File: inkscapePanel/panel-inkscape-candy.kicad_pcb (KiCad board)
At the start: 2 copper layers, 99.9 x 38.9 mm, 39 parts

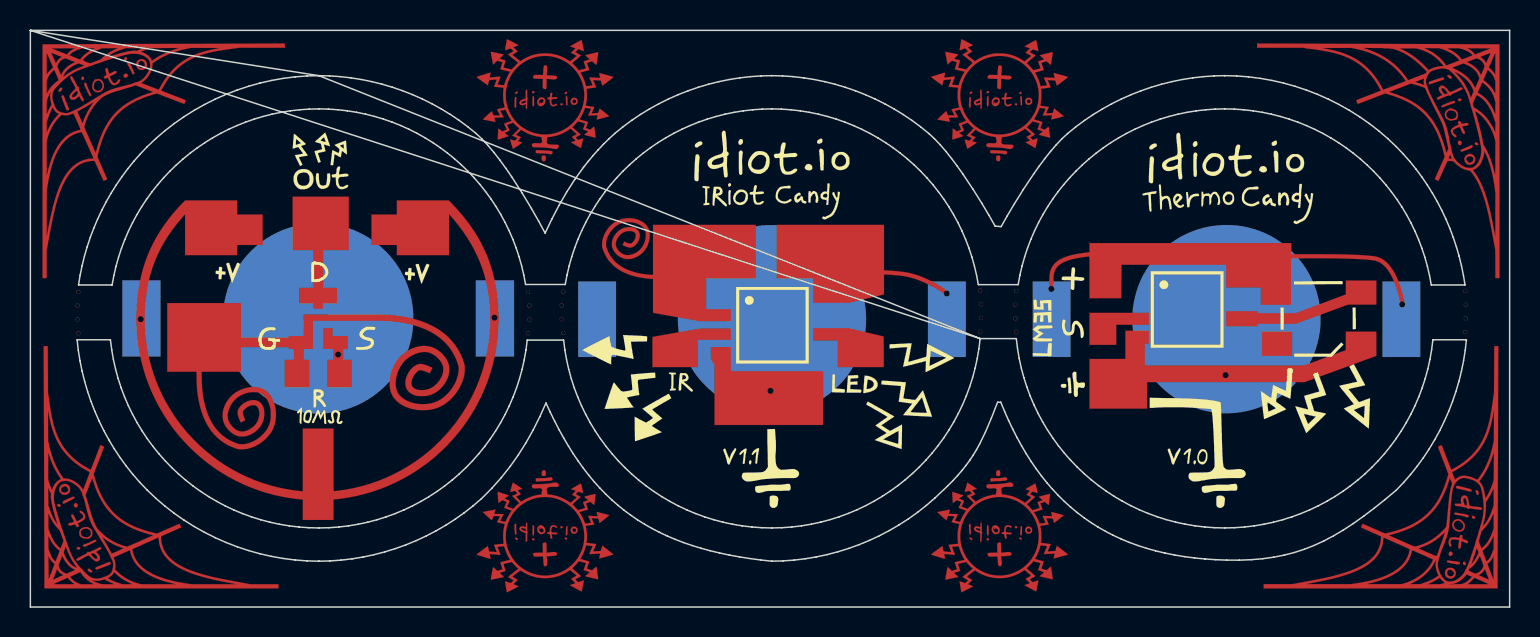
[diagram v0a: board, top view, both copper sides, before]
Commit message: new panel
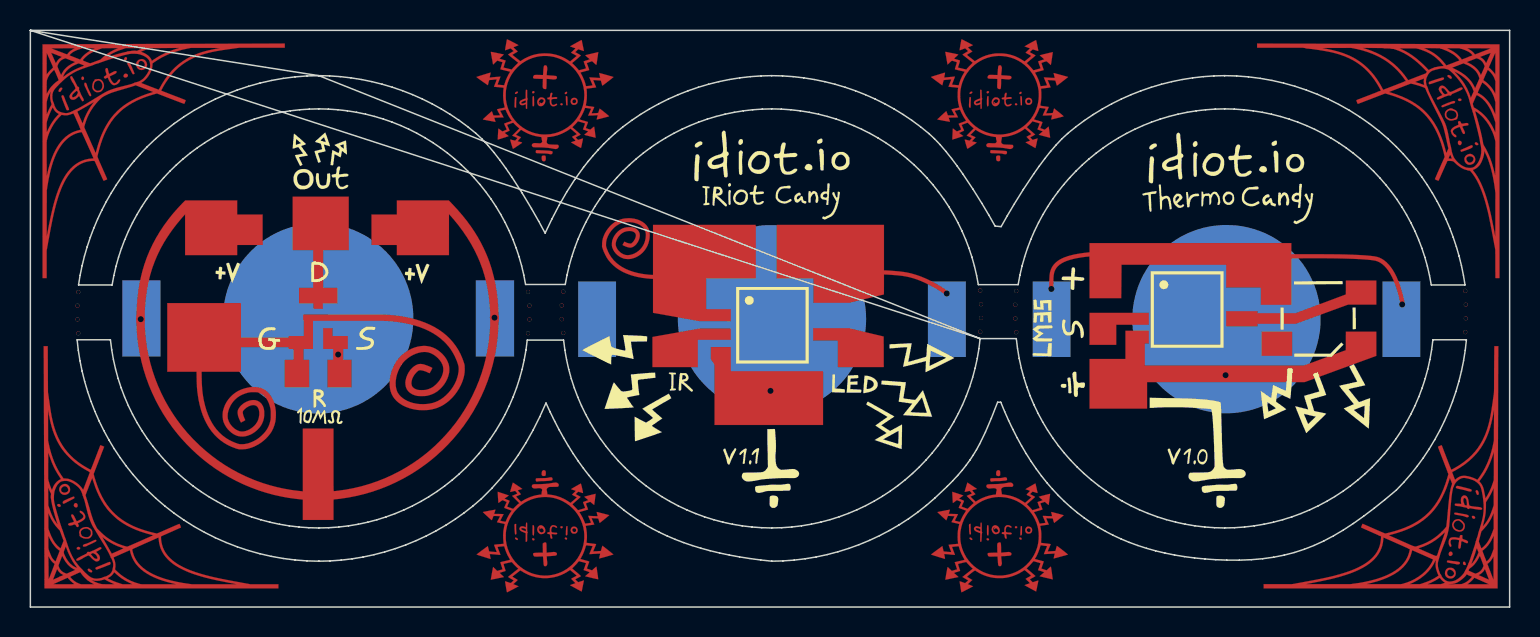
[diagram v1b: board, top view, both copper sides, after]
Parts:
- removed the G*** at (0.00, 0.00) (x6)
- added G*** (x6): LOGO, LOGO, F.Cu at (0.00, 0.00)
